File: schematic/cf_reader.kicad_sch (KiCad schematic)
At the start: 23 parts, among them J1 CF, U37 74LS245

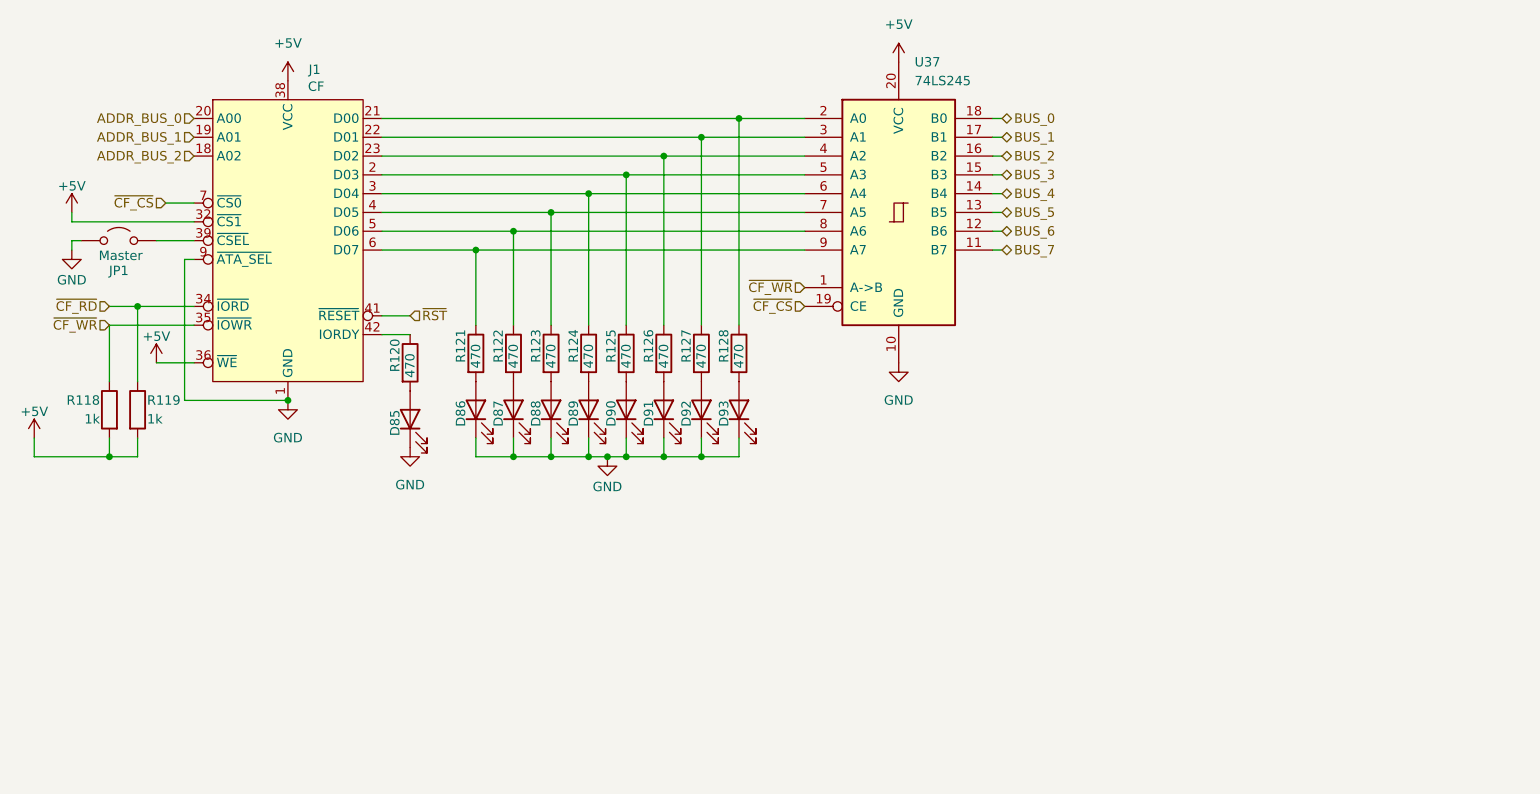
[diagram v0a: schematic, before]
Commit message: chore: update bom and footprintss
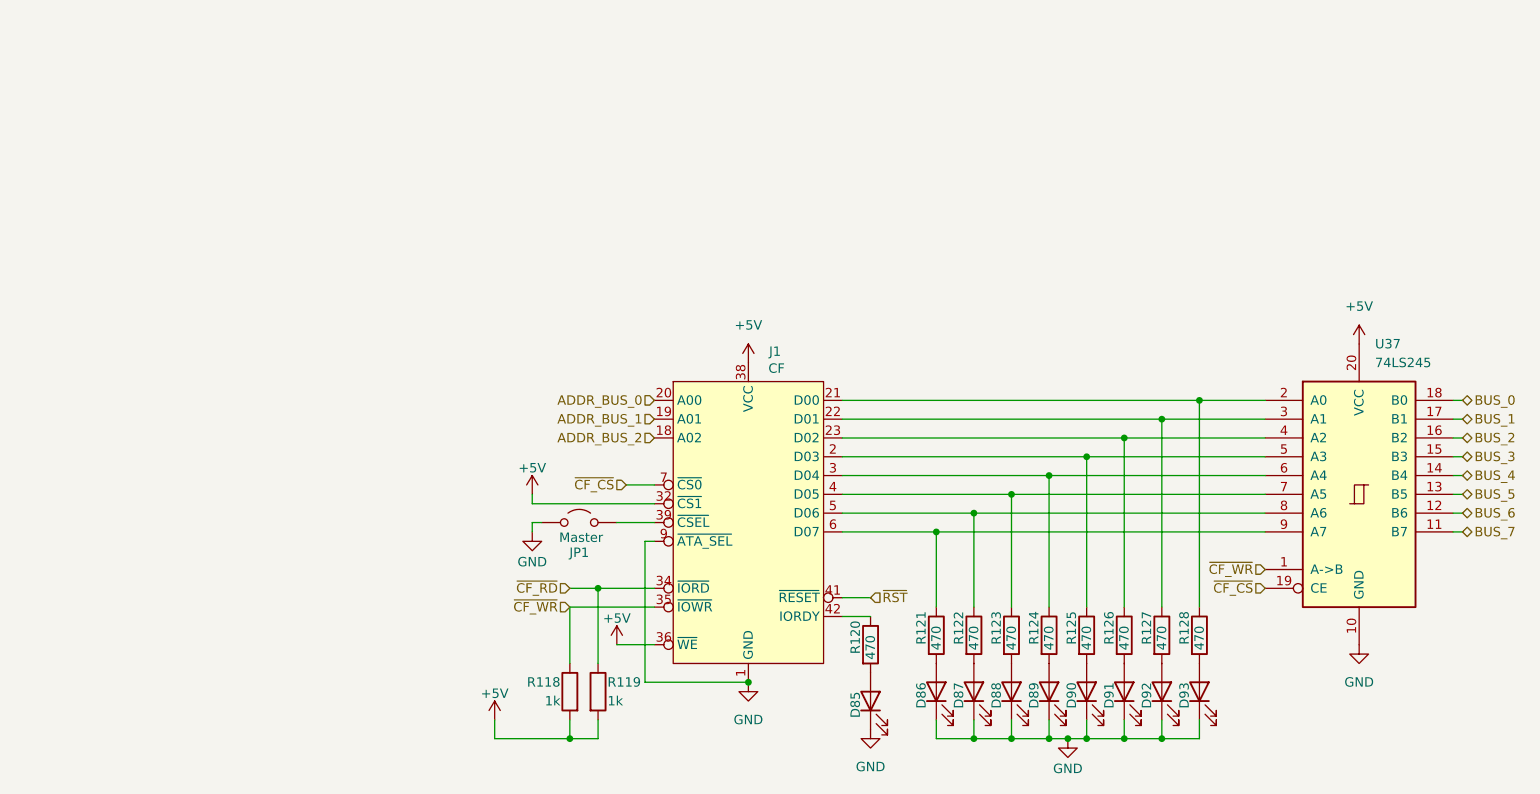
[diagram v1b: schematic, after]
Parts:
- R118, R119: footprint (none) -> Resistor_SMD:R_0805_2012Metric
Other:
- moved on the sheet: D85, D86, D87, D88, D89, D90, D91, D92, D93, J1, JP1, R118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
